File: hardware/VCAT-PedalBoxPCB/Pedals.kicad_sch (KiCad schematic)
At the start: 12 parts

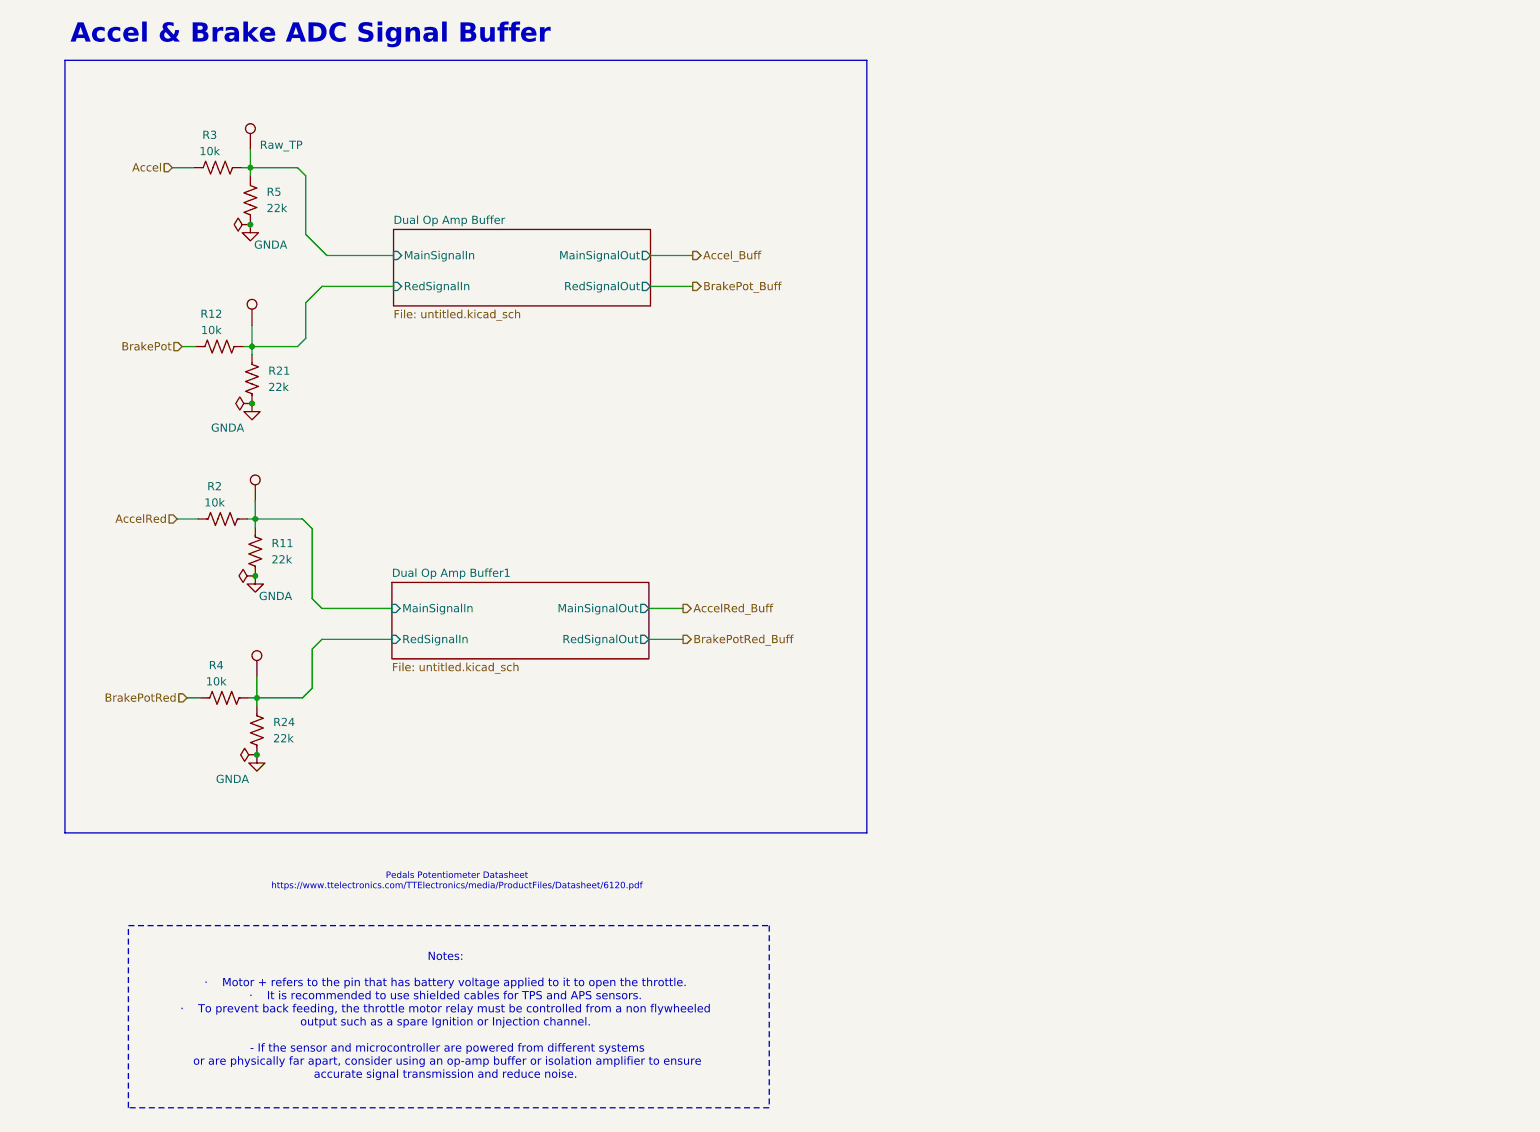
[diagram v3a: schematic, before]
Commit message: Rev B Layout #2
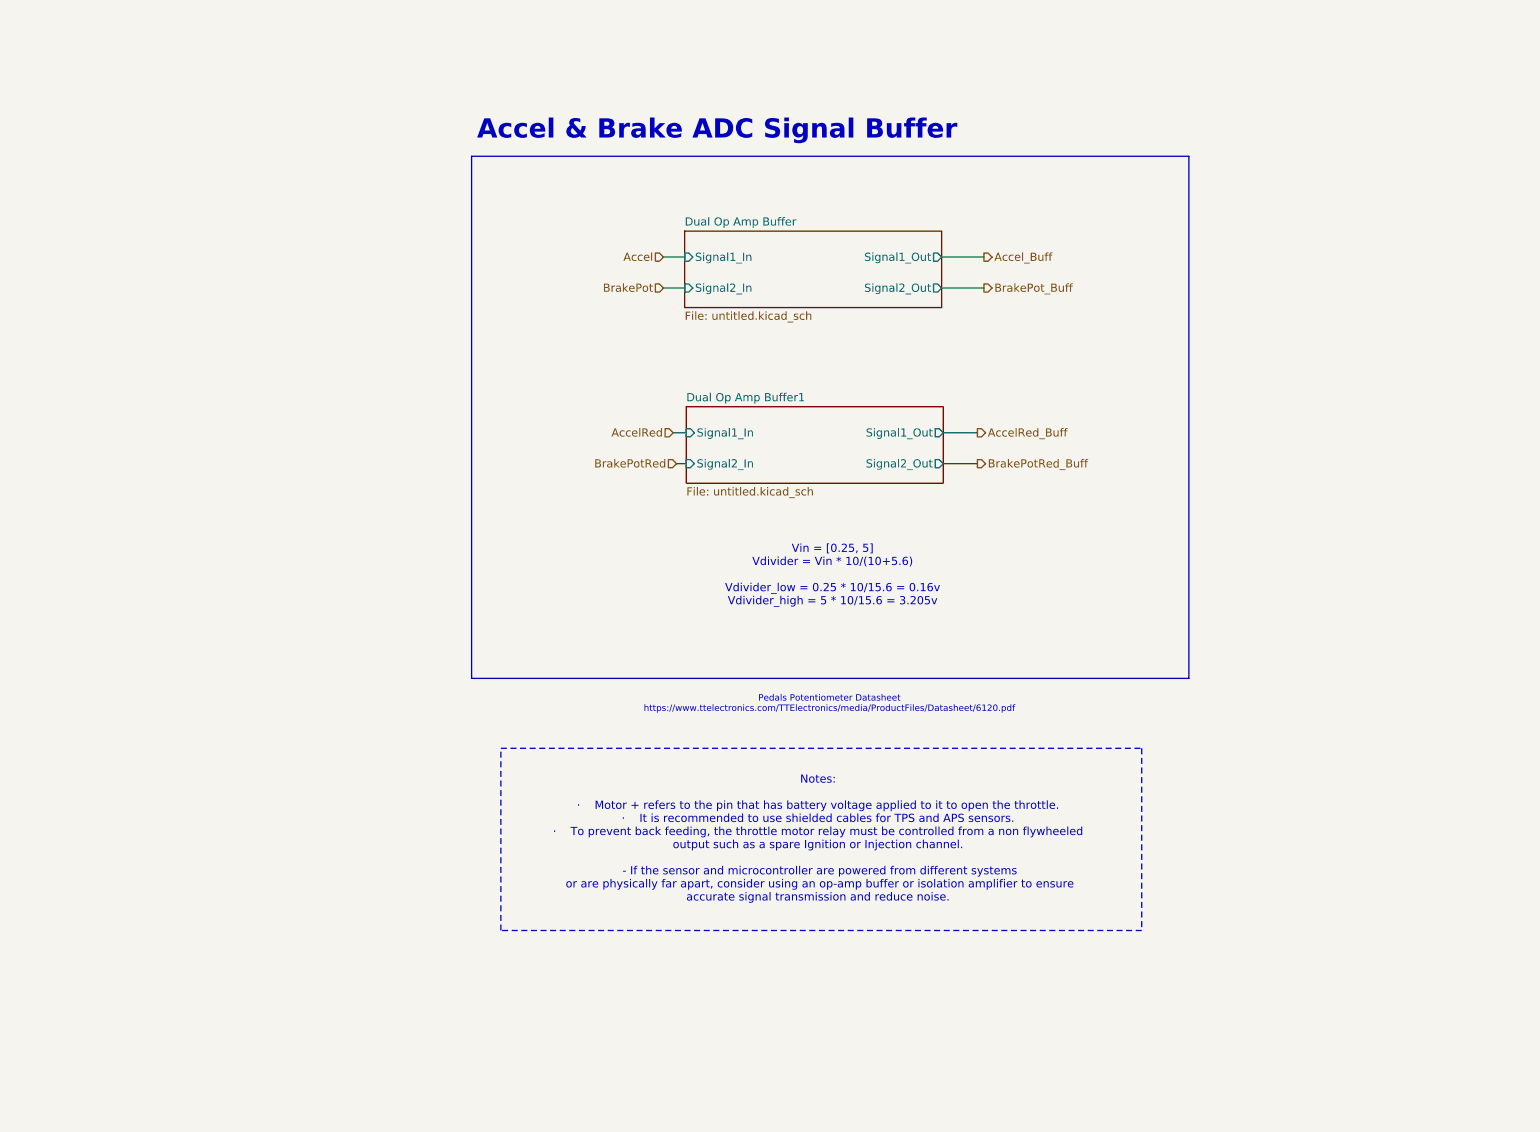
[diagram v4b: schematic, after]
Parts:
- removed AccelRaw1, AccelRaw2, BrakeRaw1, BrakeRaw2: Raw_TP, TestPoint:TestPoint_THTPad_1.5x1.5mm_Drill0.7mm, symbol Connector:TestPoint
- removed R11, R21, R24, R5: 22k, Resistor_SMD:R_0603_1608Metric_Pad0.98x0.95mm_HandSolder, symbol Device:R_US
- removed R12, R2, R3, R4: 10k, Resistor_SMD:R_0603_1608Metric_Pad0.98x0.95mm_HandSolder, symbol Device:R_US
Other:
- sheet Dual Op Amp Buffer ports: added Signal1_In, Signal1_Out, Signal2_In, Signal2_Out; removed MainSignalIn, MainSignalOut, RedSignalIn, RedSignalOut
- sheet Dual Op Amp Buffer1 ports: added Signal1_In, Signal1_Out, Signal2_In, Signal2_Out; removed MainSignalIn, MainSignalOut, RedSignalIn, RedSignalOut
- note added: "Vin = [0.25, 5] Vdivider = Vin * 10/(10+5.6) Vdivider_low = 0.25 * 10/15.6 = 0.16v Vdivider_high = 5 * 10/15.6 = 3.205v"
